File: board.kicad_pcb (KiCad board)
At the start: 2 copper layers, 92 x 72 mm, 50 parts, among them J1 LASER, J10 Mode, J11 Y, J12 12V, J13 Y, J14 X, J15 12V-36V, J16 CNC_OUT2, J2 Pololu_Breakout_A4988, J3 V_LASER, J4 Pololu_Breakout_A4988, J5 Z, J6 Pololu_Breakout_A4988, J7 12-36V, J8 Arduino_Nano, J9 Misc, K1 SRD-12VDC-SL-C, Q1 Y2, Q2 WJ0625A, T1 Logo_Open_Hardware_Small, U1 PC817, U2 XL4015E1

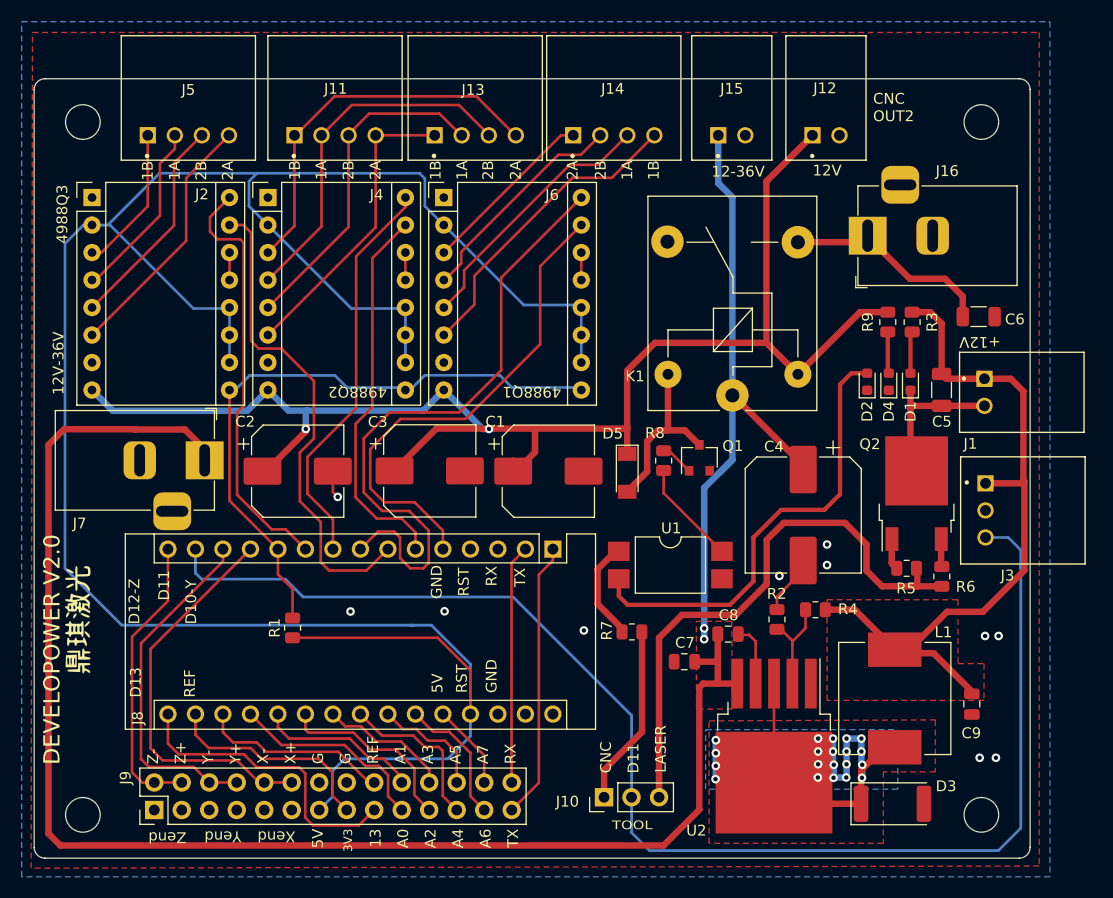
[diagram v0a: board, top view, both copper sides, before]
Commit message: Improve parts placement
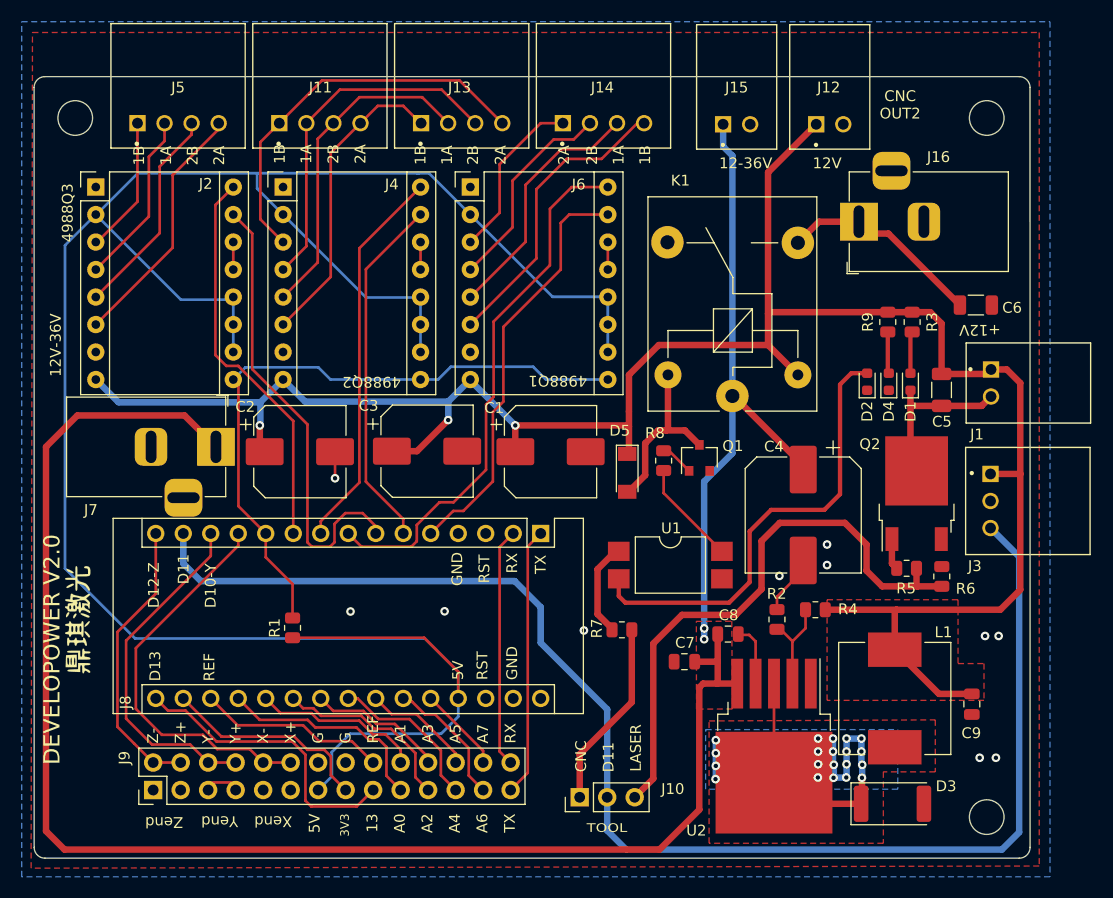
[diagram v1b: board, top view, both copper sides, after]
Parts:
- removed H3: MountingHole, MountingHole:MountingHole_3.2mm_M3
- moved J6 2.64 mm to (144.4, 73.3)
- moved J10 2.25 mm to (154.6, 129.7)
- moved J9 1.85 mm to (115.2, 129.0)
- moved C3 1.84 mm to (140.4, 97.7)
- moved J8 1.83 mm to (150.9, 105.3)
- moved C1 1.81 mm to (151.9, 97.7)
- moved C2 1.81 mm to (128.7, 97.7)
- moved J11 1.79 mm to (130.6, 67.4)
- moved J4 1.70 mm to (127.2, 73.3)
- moved J13 1.68 mm to (143.7, 67.4)
- moved J7 1.62 mm to (121.0, 97.3)
- moved J16 1.52 mm to (180.3, 76.5)
- moved J5 1.47 mm to (117.5, 67.4)
- moved J14 1.47 mm to (156.8, 67.4)
- moved J15 1.11 mm to (169.1, 67.5)
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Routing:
- net /D5: track 59.5 -> 49.8 mm
- net +12V: track 208.8 -> 199.7 mm, vias 2 -> 3
- net /D2: track 45.9 -> 38.9 mm
- net +5V: track 227.1 -> 220.3 mm
- net Net-(D3-Pad1): track 47.6 -> 44.2 mm
- net /D11: track 126.1 -> 129.3 mm
- net /D8: track 57.7 -> 60.8 mm
- net /D7: track 39.4 -> 36.3 mm
- net /D4: track 45.7 -> 43.0 mm
- net /D3: track 35.5 -> 33.0 mm
- net Net-(J14-Pad2): track 20.6 -> 19.2 mm
- net /D6: track 37.2 -> 35.8 mm
- net /A0: track 18.8 -> 20.1 mm
- net Net-(J14-Pad3): track 24.5 -> 23.3 mm
- net Net-(J11-Pad1): track 35.3 -> 36.4 mm
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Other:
- board size 92 x 72 mm -> 92 x 72.2 mm
